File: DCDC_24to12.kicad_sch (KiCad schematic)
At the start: 26 parts, among them J1 Power_IN, J2 Power_OUT, U1 BD9F800MUX-ZE2

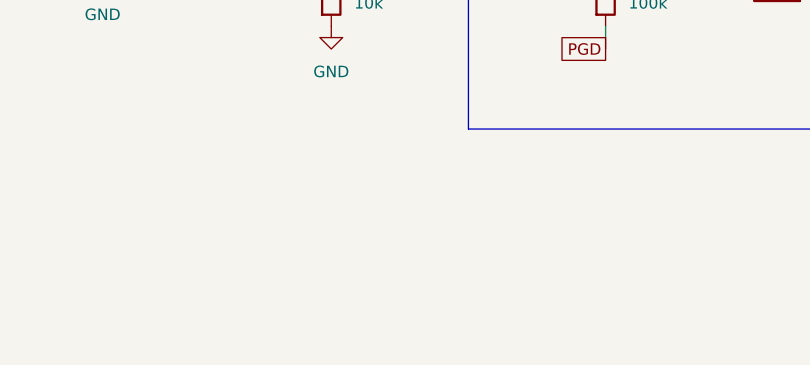
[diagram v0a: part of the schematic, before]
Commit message: 穴追加 場所がねぇ
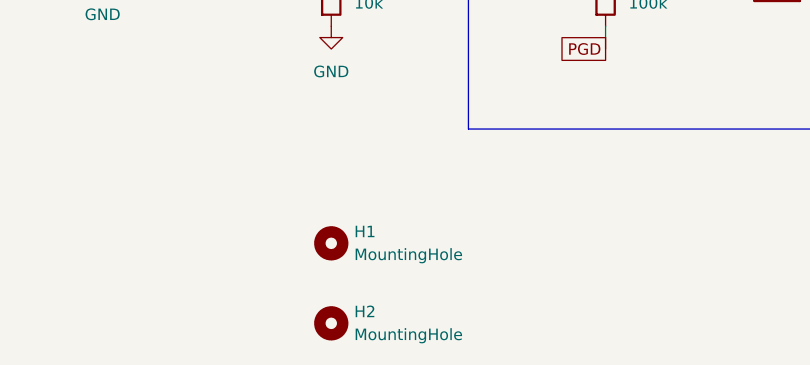
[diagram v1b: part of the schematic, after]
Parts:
- added H1, H2: MountingHole, MountingHole:MountingHole_3.2mm_M3_Pad_Via, symbol Mechanical:MountingHole
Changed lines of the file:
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@@
+	)
+	(symbol
+		(lib_id "Mechanical:MountingHole")
+		(at 71.12 166.37 0)
+		(unit 1)
+		(exclude_from_sim yes)
+		(in_bom no)
+		(on_board yes)
+		(dnp no)
+		(fields_autoplaced yes)
+		(property "Reference" "H2"
+			(at 73.66 165.0999 0)
+			(effects
+				(font
+					(size 1.27 1.27)
+				)
+				(justify left)
+			)
+		)
+		(property "Value" "MountingHole"
+			(at 73.66 167.6399 0)
+			(effects
+				(font
+					(size 1.27 1.27)
+				)
+				(justify left)
+			)
+		)
+		(property "Footprint" "MountingHole:MountingHole_3.2mm_M3_Pad_Via"
+			(at 71.12 166.37 0)
+			(effects
+				(font
+					(size 1.27 1.27)
+				)
+				(hide yes)
+			)
+		)
+		(property "Datasheet" "~"
+			(at 71.12 166.37 0)
+			(effects
+				(font
+					(size 1.27 1.27)
+				)
+				(hide yes)
+			)
+		)
+		(property "Description" "Mounting Hole without connection"
+			(at 71.12 166.37 0)
+			(effects
+				(font
+					(size 1.27 1.27)
+				)
+				(hide yes)
+			)
+		)
+		(instances
+			(project ""
+				(path "/9b31bb12-b0a4-46c2-8fe3-73cecf9f3124"
+					(reference "H2")
+					(unit 1)
+				)
+			)
+		)
 	)
 	(symbol
@@
 					(unit 1)
 				)
+			)
+		)
+	)
+	(symbol
+		(lib_id "Mechanical:MountingHole")
+		(at 71.12 157.48 0)
+		(unit 1)
+		(exclude_from_sim yes)
+		(in_bom no)
+		(on_board yes)
+		(dnp no)
+		(fields_autoplaced yes)
+		(property "Reference" "H1"
+			(at 73.66 156.2099 0)
+			(effects
+				(font
+					(size 1.27 1.27)
+				)
+				(justify left)
+			)
+		)
+		(property "Value" "MountingHole"
+			(at 73.66 158.7499 0)
+			(effects
+				(font
+					(size 1.27 1.27)
+				)
+				(justify left)
+			)
+		)
+		(property "Footprint" "MountingHole:MountingHole_3.2mm_M3_Pad_Via"
+			(at 71.12 157.48 0)
+			(effects
+				(font
+					(size 1.27 1.27)
+				)
+				(hide yes)
+			)
+		)
+		(property "Datasheet" "~"
+			(at 71.12 157.48 0)
+			(effects
+				(font
+					(size 1.27 1.27)
+				)
+				(hide yes)
+			)
+		)
+		(property "Description" "Mounting Hole without connection"
+			(at 71.12 157.48 0)
+			(effects
+				(font
+					(size 1.27 1.27)
+				)
+				(hide yes)
+			)
+		)
+		(instances
+			(project ""
+				(path "/9b31bb12-b0a4-46c2-8fe3-73cecf9f3124"
+					(reference "H1")
+					(unit 1)
+				)
